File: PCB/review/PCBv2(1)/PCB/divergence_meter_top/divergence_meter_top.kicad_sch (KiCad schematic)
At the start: 14 parts

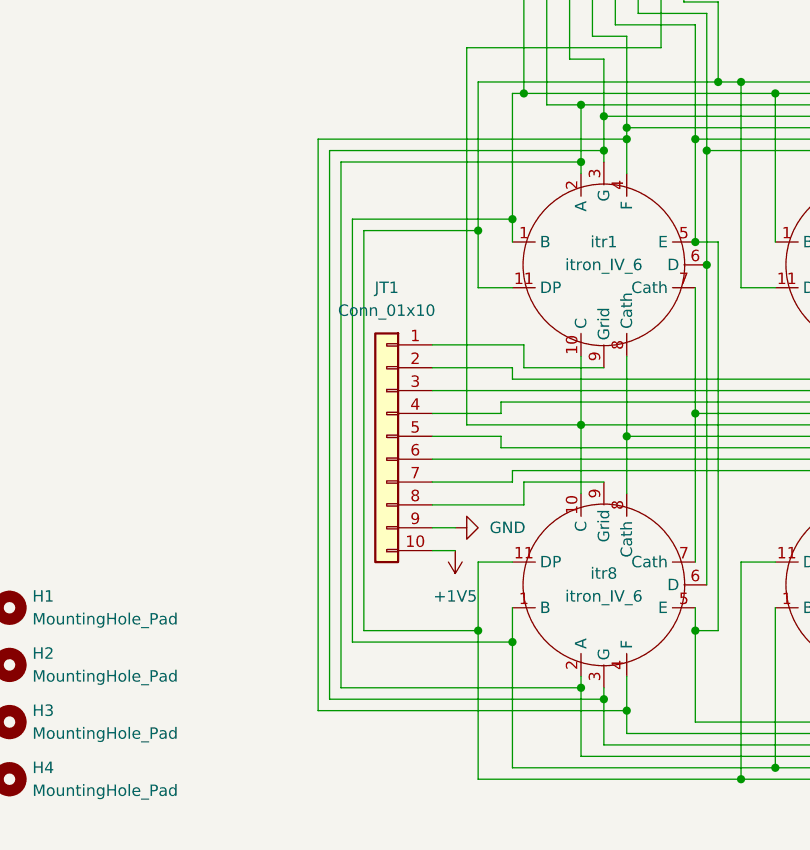
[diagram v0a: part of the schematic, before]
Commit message: reviewing top board
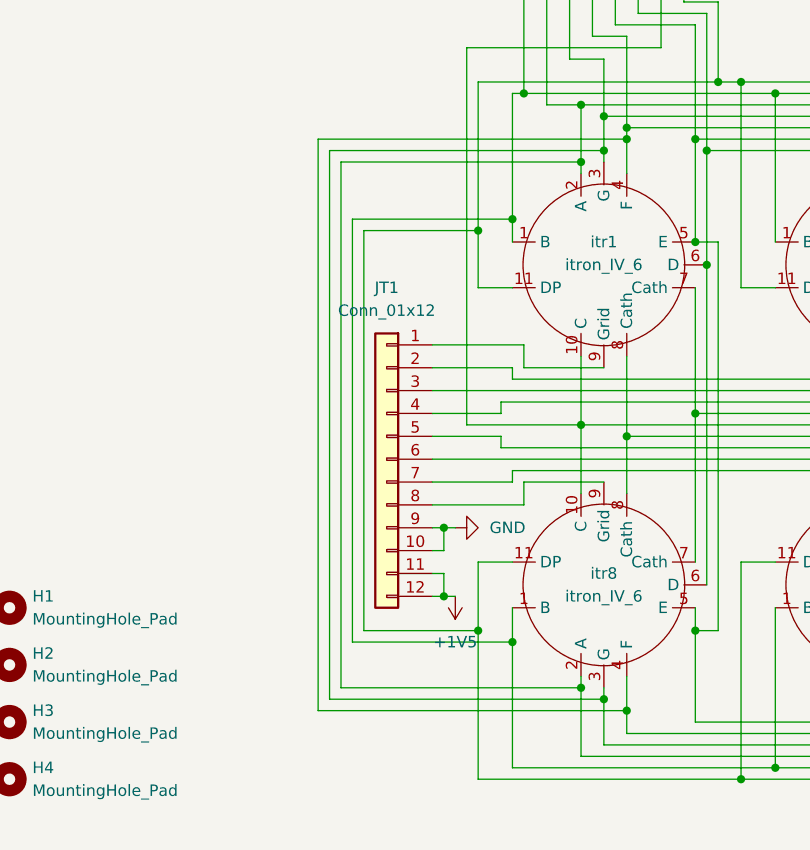
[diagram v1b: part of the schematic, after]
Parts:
- removed JT1: Conn_01x10, Connector_PinHeader_2.54mm:PinHeader_1x10_P2.54mm_Vertical, symbol Connector_Generic:Conn_01x10
- added JT1: Conn_01x12, Connector_PinHeader_2.54mm:PinHeader_1x12_P2.54mm_Vertical, symbol Connector_Generic:Conn_01x12
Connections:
- net +1V5: now also JT1.11 (Pin_11), JT1.12 (Pin_12)
- net GND: now also JT1.10 (Pin_10), JT1.9 (Pin_9)
- net at itr1.9 (Grid): now also JT1.1 (Pin_1)
- net at itr2.9 (Grid): now also JT1.2 (Pin_2)
- net at itr3.9 (Grid): now also JT1.3 (Pin_3)
- net at itr4.9 (Grid): now also JT1.4 (Pin_4)
- net at itr5.9 (Grid): now also JT1.5 (Pin_5)
- net at itr6.9 (Grid): now also JT1.6 (Pin_6)
- net at itr7.9 (Grid): now also JT1.7 (Pin_7)
- net at itr8.9 (Grid): now also JT1.8 (Pin_8)
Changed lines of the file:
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@@
   (junction (at 149.86 101.6) (diameter 0) (color 0 0 0 0)
   )
+  (junction (at 105.41 120.65) (diameter 0) (color 0 0 0 0)
+  )
   (junction (at 120.65 72.39) (diameter 0) (color 0 0 0 0)
   )
@@
   (junction (at 181.61 68.58) (diameter 0) (color 0 0 0 0)
   )
+  (junction (at 105.41 113.03) (diameter 0) (color 0 0 0 0)
+  )
   (junction (at 120.65 130.81) (diameter 0) (color 0 0 0 0)
   )
@@
     (stroke (width 0) (type default) (color 0 0 0 0))
   )
-  (wire (pts (xy 93.98 130.81) (xy 93.98 72.39))
-    (stroke (width 0) (type default) (color 0 0 0 0))
-  )
   (wire (pts (xy 181.61 102.87) (xy 208.28 102.87))
     (stroke (width 0) (type default) (color 0 0 0 0))
@@
     (stroke (width 0) (type default) (color 0 0 0 0))
   )
+  (wire (pts (xy 105.41 120.65) (xy 106.68 120.65))
+    (stroke (width 0) (type default) (color 0 0 0 0))
+  )
   (wire (pts (xy 189.23 69.85) (xy 215.9 69.85))
     (stroke (width 0) (type default) (color 0 0 0 0))
@@
     (stroke (width 0) (type default) (color 0 0 0 0))
   )
-  (wire (pts (xy 104.14 113.03) (xy 106.68 113.03))
+  (wire (pts (xy 104.14 113.03) (xy 105.41 113.03))
     (stroke (width 0) (type default) (color 0 0 0 0))
   )
@@
     (stroke (width 0) (type default) (color 0 0 0 0))
   )
+  (wire (pts (xy 105.41 118.11) (xy 105.41 120.65))
+    (stroke (width 0) (type default) (color 0 0 0 0))
+  )
   (wire (pts (xy 114.3 64.77) (xy 142.24 64.77))
     (stroke (width 0) (type default) (color 0 0 0 0))
@@
     (stroke (width 0) (type default) (color 0 0 0 0))
   )
+  (wire (pts (xy 105.41 113.03) (xy 106.68 113.03))
+    (stroke (width 0) (type default) (color 0 0 0 0))
+  )
   (wire (pts (xy 217.17 83.82) (xy 217.17 119.38))
     (stroke (width 0) (type default) (color 0 0 0 0))
@@
     (stroke (width 0) (type default) (color 0 0 0 0))
   )
+  (wire (pts (xy 104.14 118.11) (xy 105.41 118.11))
+    (stroke (width 0) (type default) (color 0 0 0 0))
+  )
   (wire (pts (xy 138.43 86.36) (xy 142.24 86.36))
     (stroke (width 0) (type default) (color 0 0 0 0))
   )
+  (wire (pts (xy 93.98 72.39) (xy 93.98 130.81))
+    (stroke (width 0) (type default) (color 0 0 0 0))
+  )
   (wire (pts (xy 120.65 138.43) (xy 149.86 138.43))
     (stroke (width 0) (type default) (color 0 0 0 0))
   )
+  (wire (pts (xy 104.14 115.57) (xy 105.41 115.57))
+    (stroke (width 0) (type default) (color 0 0 0 0))
+  )
   (wire (pts (xy 104.14 105.41) (xy 179.07 105.41))
     (stroke (width 0) (type default) (color 0 0 0 0))
@@
     (stroke (width 0) (type default) (color 0 0 0 0))
   )
-  (wire (pts (xy 104.14 115.57) (xy 106.68 115.57))
-    (stroke (width 0) (type default) (color 0 0 0 0))
-  )
-  (symbol (lib_id "power:+1V5") (at 106.68 115.57 180) (unit 1)
+  (wire (pts (xy 104.14 120.65) (xy 105.41 120.65))
+    (stroke (width 0) (type default) (color 0 0 0 0))
+  )
+  (wire (pts (xy 105.41 115.57) (xy 105.41 113.03))
+    (stroke (width 0) (type default) (color 0 0 0 0))
+  )
+  (symbol (lib_id "power:+1V5") (at 106.68 120.65 180) (unit 1)
     (in_bom yes) (on_board yes) (fields_autoplaced)
-    (property "Reference" "#PWR0104" (id 0) (at 106.68 111.76 0)
-      (effects (font (size 1.27 1.27)) hide)
-    )
-    (property "Value" "+1V5" (id 1) (at 106.68 120.65 0))
-    (property "Footprint" "" (id 2) (at 106.68 115.57 0)
-      (effects (font (size 1.27 1.27)) hide)
-    )
-    (property "Datasheet" "" (id 3) (at 106.68 115.57 0)
-      (effects (font (size 1.27 1.27)) hide)
-    )
-    (pin "1")
-  )
-  (symbol (lib_id "Connector_Generic:Conn_01x10") (at 99.06 102.87 0) (mirror y) (unit 1)
-    (in_bom yes) (on_board yes) (fields_autoplaced)
-    (property "Reference" "JT1" (id 0) (at 99.06 86.36 0))
-    (property "Value" "Conn_01x10" (id 1) (at 99.06 88.9 0))
-    (property "Footprint" "Connector_PinHeader_2.54mm:PinHeader_1x10_P2.54mm_Vertical" (id 2) (at 99.06 102.87 0)
-      (effects (font (size 1.27 1.27)) hide)
-    )
-    (property "Datasheet" "~" (id 3) (at 99.06 102.87 0)
-      (effects (font (size 1.27 1.27)) hide)
-    )
-    (pin "1")
-    (pin "10")
-    (pin "2")
-    (pin "3")
-    (pin "4")
-    (pin "5")
-    (pin "6")
-    (pin "7")
-    (pin "8")
-    (pin "9")
+    (property "Reference" "#PWR0104" (id 0) (at 106.68 116.84 0)
+      (effects (font (size 1.27 1.27)) hide)
+    )
+    (property "Value" "+1V5" (id 1) (at 106.68 125.73 0))
+    (property "Footprint" "" (id 2) (at 106.68 120.65 0)
+      (effects (font (size 1.27 1.27)) hide)
+    )
+    (property "Datasheet" "" (id 3) (at 106.68 120.65 0)
+      (effects (font (size 1.27 1.27)) hide)
+    )
+    (pin "1")
   )
   (symbol (lib_id "itron_iv_6:itron_IV_6") (at 123.19 69.85 0) (unit 1)
@@
   (symbol (lib_id "power:GND") (at 53.34 148.59 0) (unit 1)
     (in_bom yes) (on_board yes)
-    (property "Reference" "#PWR?" (id 0) (at 53.34 154.94 0)
+    (property "Reference" "#PWR0105" (id 0) (at 53.34 154.94 0)
       (effects (font (size 1.27 1.27)) hide)
     )
@@
   (symbol (lib_id "power:GND") (at 222.25 100.33 90) (unit 1)
     (in_bom yes) (on_board yes) (fields_autoplaced)
-    (property "Reference" "#PWR?" (id 0) (at 228.6 100.33 0)
+    (property "Reference" "#PWR0101" (id 0) (at 228.6 100.33 0)
       (effects (font (size 1.27 1.27)) hide)
     )
@@
   (symbol (lib_id "power:GND") (at 106.68 113.03 90) (unit 1)
     (in_bom yes) (on_board yes) (fields_autoplaced)
-    (property "Reference" "#PWR?" (id 0) (at 113.03 113.03 0)
+    (property "Reference" "#PWR0103" (id 0) (at 113.03 113.03 0)
       (effects (font (size 1.27 1.27)) hide)
     )
@@
     (pin "9")
   )
+  (symbol (lib_id "Connector_Generic:Conn_01x12") (at 99.06 105.41 0) (mirror y) (unit 1)
+    (in_bom yes) (on_board yes) (fields_autoplaced)
+    (property "Reference" "JT1" (id 0) (at 99.06 86.36 0))
+    (property "Value" "Conn_01x12" (id 1) (at 99.06 88.9 0))
+    (property "Footprint" "Connector_PinHeader_2.54mm:PinHeader_1x12_P2.54mm_Vertical" (id 2) (at 99.06 105.41 0)
+      (effects (font (size 1.27 1.27)) hide)
+    )
+    (property "Datasheet" "~" (id 3) (at 99.06 105.41 0)
+      (effects (font (size 1.27 1.27)) hide)
+    )
+    (pin "1")
+    (pin "10")
+    (pin "11")
+    (pin "12")
+    (pin "2")
+    (pin "3")
+    (pin "4")
+    (pin "5")
+    (pin "6")
+    (pin "7")
+    (pin "8")
+    (pin "9")
+  )
   (symbol (lib_id "itron_iv_6:itron_IV_6") (at 152.4 133.35 0) (mirror x) (unit 1)
     (in_bom yes) (on_board yes)
@@
   )
   (symbol_instances
+    (path "/791d115a-50b3-4488-9597-daa84ef7a043"
+      (reference "#PWR0101") (unit 1) (value "GND") (footprint "")
+    )
     (path "/67f0fb9a-0f63-43d9-89e2-b6a97dc8e6af"
       (reference "#PWR0102") (unit 1) (value "+1V5") (footprint "")
     )
+    (path "/88fbee1a-2719-4ce6-98b9-473040b84750"
+      (reference "#PWR0103") (unit 1) (value "GND") (footprint "")
+    )
     (path "/01bb07b7-5eda-4da8-b61b-2d6248635b61"
       (reference "#PWR0104") (unit 1) (value "+1V5") (footprint "")
     )
     (path "/376d7c50-6080-4e30-a4e6-806d032cc07c"
-      (reference "#PWR?") (unit 1) (value "GND") (footprint "")
-    )
-    (path "/791d115a-50b3-4488-9597-daa84ef7a043"
-      (reference "#PWR?") (unit 1) (value "GND") (footprint "")
-    )
-    (path "/88fbee1a-2719-4ce6-98b9-473040b84750"
-      (reference "#PWR?") (unit 1) (value "GND") (footprint "")
+      (reference "#PWR0105") (unit 1) (value "GND") (footprint "")
     )
     (path "/959049d5-8131-4d90-90cb-f74b567fc392"
@@
       (reference "H4") (unit 1) (value "MountingHole_Pad") (footprint "MountingHole:MountingHole_3.5mm_Pad_Via")
     )
-    (path "/1a55f54c-7f6f-4392-b020-7d75fd2b3fb5"
-      (reference "JT1") (unit 1) (value "Conn_01x10") (footprint "Connector_PinHeader_2.54mm:PinHeader_1x10_P2.54mm_Vertical")
+    (path "/e35b130e-f843-46e9-acbf-8b5ba0b2103d"
+      (reference "JT1") (unit 1) (value "Conn_01x12") (footprint "Connector_PinHeader_2.54mm:PinHeader_1x12_P2.54mm_Vertical")
     )
     (path "/ab4e121c-071f-4432-a221-b67e64d6ff8d"
